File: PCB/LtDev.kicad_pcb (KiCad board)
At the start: 2 copper layers, 90 x 50 mm, 113 parts, among them IC1 TMUX1134PWR, IC2 MMS9013-H-TP, IC3 TPS2116DRLR, IC4 TPS2116DRLR, J1 Conn_JTAG_02x07, J2 Conn_02x05_Odd_Even, J3 Conn_02x05_Odd_Even, J4 Screw_Terminal_01x02, J5 Conn_01x04_Pin, J7 Conn_01x06_Pin, J9 Jumper_Pin_ VIO_CP&3V3, P1 USB_C_Plug (Conv), P2 USB_C_Plug (Prog), SW1 SW_DIP_x02, SW2 SW_DIP_x02, SW3 SW_Push, U1 AMS1117, U2 AMS1117, U3 STM32F103CBTx, U4 CP2102N-Axx-xQFN24, Y1 8MHz

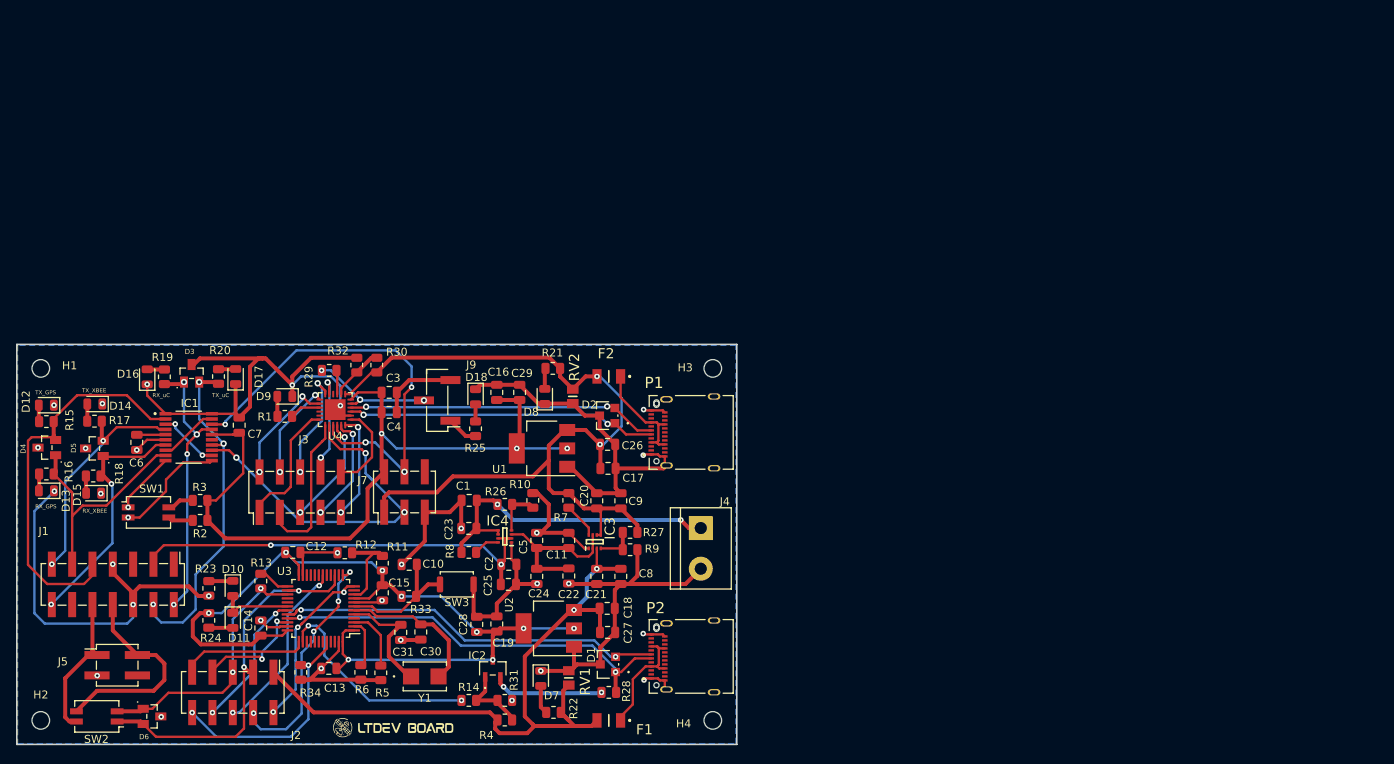
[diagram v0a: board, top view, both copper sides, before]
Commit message: Add files via upload
1.1.0
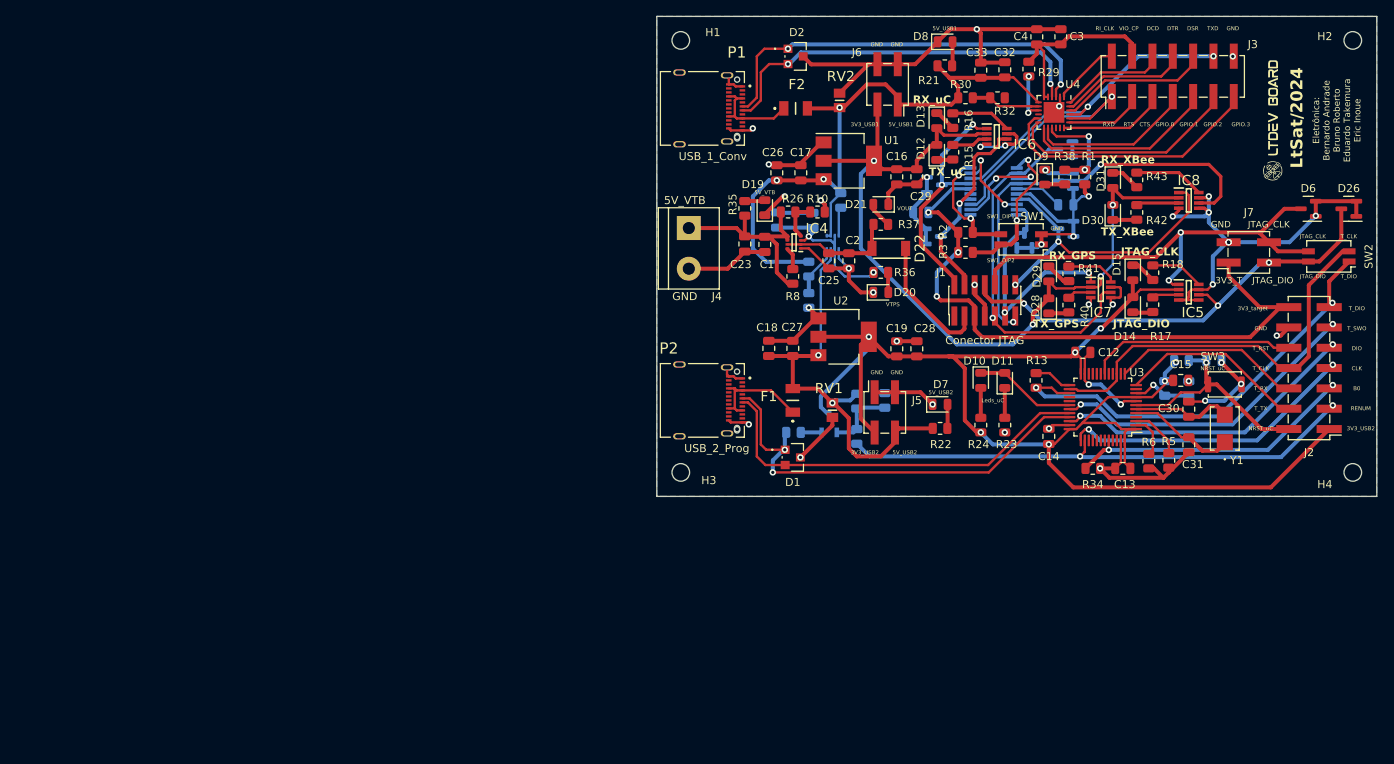
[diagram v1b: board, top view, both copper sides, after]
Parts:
- removed C20, C21, C24: 10uF, Capacitor_SMD:C_0805_2012Metric
- removed C5, C8, C9: 100nF, Capacitor_SMD:C_0805_2012Metric
- removed D16, D17: LED_Green, LED_SMD:LED_0805_2012Metric
- removed D18: LED_Yellow, LED_SMD:LED_0805_2012Metric
- removed J9: Jumper_Pin_ VIO_CP&3V3, Connector_PinHeader_2.54mm:PinHeader_1x03_P2.54mm_Vertical_SMD_Pin1Left
- removed R19, R20: 100R, Resistor_SMD:R_0805_2012Metric
- removed R25: 220R, Resistor_SMD:R_0805_2012Metric
- added C32: 100nF, Capacitor_SMD:C_0805_2012Metric, F.Cu at (179.0, 36.7)
- added C33: 4.7uF, Capacitor_SMD:C_0805_2012Metric, F.Cu at (176.0, 36.7)
- added D19: LED_Red, LED_SMD:LED_0805_2012Metric, F.Cu at (149.0, 53.9)
- added D20: LED_Red, LED_SMD:LED_0805_2012Metric, F.Cu at (163.5, 64.5)
- added D21: LED_Red, LED_SMD:LED_0805_2012Metric, F.Cu at (163.5, 53.5)
- added D22: CMS04_TE12L,Q,M_, Lt_Dev:SODFL4724X108N, F.Cu at (164.5, 59.0)
- added D23: SLVU2.8-MS, Package_TO_SOT_SMD:SOT-23, B.Cu at (186.6, 56.5)
- added D24: SLVU2.8-MS, Package_TO_SOT_SMD:SOT-23, B.Cu at (186.6, 50.5)
- added D25: SLVU2.8-MS, Package_TO_SOT_SMD:SOT-23, B.Cu at (186.5, 46.6)
- added D26: SLVU2.8-MS, Package_TO_SOT_SMD:SOT-23, F.Cu at (222.0, 54.0)
- added D28: LED_Green, LED_SMD:LED_0805_2012Metric, F.Cu at (184.5, 66.2)
- added D29: LED_Green, LED_SMD:LED_0805_2012Metric, F.Cu at (184.5, 62.2)
- added D30: LED_Green, LED_SMD:LED_0805_2012Metric, F.Cu at (192.5, 54.5)
- added D31: LED_Green, LED_SMD:LED_0805_2012Metric, F.Cu at (192.5, 50.5)
- added IC5: TS3A4742DCNR, Lt_Dev:SOT65P280X145-8N, F.Cu at (202.0, 64.5)
- added IC6: TS3A4741DCNR, Lt_Dev:SOT65P280X145-8N, F.Cu at (178.0, 45.0)
- added IC7: TS3A4741DCNR, Lt_Dev:SOT65P280X145-8N, F.Cu at (191.0, 64.2)
- added IC8: TS3A4741DCNR, Lt_Dev:SOT65P280X145-8N, F.Cu at (202.0, 53.0)
- added J6: Conn_02x02_Odd_Even, Connector_PinSocket_2.54mm:PinSocket_2x02_P2.54mm_Vertical_SMD, F.Cu at (164.3, 38.5)
- added R35: 120R, Resistor_SMD:R_0805_2012Metric, F.Cu at (146.5, 54.0)
- added R36: 120R, Resistor_SMD:R_0805_2012Metric, F.Cu at (163.5, 62.0)
- added R37: 120R, Resistor_SMD:R_0805_2012Metric, F.Cu at (163.5, 56.0)
- added R38: 100R, Resistor_SMD:R_0805_2012Metric, F.Cu at (186.5, 50.1)
- added R40: 100R, Resistor_SMD:R_0805_2012Metric, F.Cu at (187.0, 66.1)
- added R41: 100R, Resistor_SMD:R_0805_2012Metric, F.Cu at (187.0, 62.2)
- added R42: 100R, Resistor_SMD:R_0805_2012Metric, F.Cu at (195.5, 54.5)
- added R43: 100R, Resistor_SMD:R_0805_2012Metric, F.Cu at (195.5, 50.4)
- C10, C11, C22, C6, C7, IC1, IC2, IC3, R11, R12, R14, R27, R28, R31, R33, R4, R7, R9: moved to B.Cu
- C4: value 100nF -> 4.7uF
- D10, D9: value LED_Red -> LED_Yellow
- D11: value LED_Yellow -> LED_Red
- D3, D4, D5: value PESD3V3S2UAT,215 -> SLVU2.8-MS; footprint Lt_Dev:SOT95P230X110-3N -> Package_TO_SOT_SMD:SOT-23; moved to B.Cu
- D6: value PESD3V3S2UAT,215 -> SLVU2.8-MS; footprint Lt_Dev:SOT95P230X110-3N -> Package_TO_SOT_SMD:SOT-23
- J1: footprint Connector_PinHeader_2.54mm:PinHeader_2x07_P2.54mm_Vertical_SMD -> Connector_PinHeader_1.27mm:PinHeader_2x07_P1.27mm_Vertical_SMD
- J2, J3: value Conn_02x05_Odd_Even -> Conn_JTAG_02x07; footprint Connector_PinHeader_2.54mm:PinHeader_2x05_P2.54mm_Vertical_SMD -> Connector_PinHeader_2.54mm:PinHeader_2x07_P2.54mm_Vertical_SMD
- J5: value Conn_01x04_Pin -> Conn_02x02_Odd_Even; footprint Connector_PinHeader_2.54mm:PinHeader_2x02_P2.54mm_Vertical_SMD -> Connector_PinSocket_2.54mm:PinSocket_2x02_P2.54mm_Vertical_SMD
- J7: value Conn_01x06_Pin -> Conn_02x02_Odd_Even; footprint Connector_PinHeader_2.54mm:PinHeader_2x03_P2.54mm_Vertical_SMD -> Connector_PinSocket_2.54mm:PinSocket_2x02_P2.54mm_Vertical_SMD
- R29: value 2k -> 1k
- moved H2 184.7 mm to (222.5, 33.0)
- moved SW2 164.4 mm to (219.5, 60.0)
- moved D6 157.9 mm to (216.9, 54.0), turned to 180 degrees
- moved J2 140.5 mm to (217.0, 74.0), turned to 180 degrees
- moved R18 134.9 mm to (197.5, 62.0), turned to 90 degrees
- moved G*** 133.7 mm to (212.5, 43.5), turned to 90 degrees
- moved R17 133.1 mm to (197.5, 66.0), turned to 90 degrees
- moved D15 132.8 mm to (195.0, 62.0), turned to -90 degrees
- moved D14 130.3 mm to (195.0, 66.0), turned to 90 degrees
- moved R16 121.6 mm to (172.5, 43.0), turned to 90 degrees
- moved J3 120.8 mm to (200.0, 37.5)
- moved D13 120.5 mm to (170.5, 43.0), turned to -90 degrees
- moved C6 119.9 mm to (186.6, 53.5), turned to 0 degrees
- moved D5 119.1 mm to (181.4, 58.0)
- moved R15 118.2 mm to (172.5, 47.0), turned to 90 degrees
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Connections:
- C10 pad 1: /NRST -> /NRST_uC
- C3 pad 1: /3V3_USB1 -> /VIO_CP
- C3 pad 2: Net-(J9-Pin_3) -> GND
- C4 pad 1: /3V3_USB1 -> /VIO_CP
- C4 pad 2: Net-(J9-Pin_3) -> GND
- C7 pad 1: /3V3_USB1 -> /3V3_target
- D10 pad 1: Net-(D10-K) -> /LED
- D10 pad 2: /LED -> Net-(D10-A)
- D11 pad 1: /LED -> Net-(D11-K)
- D11 pad 2: Net-(D11-A) -> /LED
- D12 pad 1: GND -> Net-(D12-K)
- D12 pad 2: Net-(D12-A) -> /3V3_USB1
- D13 pad 1: GND -> Net-(D13-K)
- D13 pad 2: Net-(D13-A) -> /3V3_USB1
- D14 pad 1: GND -> Net-(D14-K)
- D14 pad 2: Net-(D14-A) -> /3V3_USB2
- D15 pad 1: GND -> Net-(D15-K)
- D15 pad 2: Net-(D15-A) -> /3V3_USB2
- D3 pad 1: /RX_uC -> GND
- D3 pad 2: /TX_uC -> GND
- D3 pad 3: GND -> /RX_uC
- D4 pad 1: /RX_GPS -> GND
- D4 pad 2: /TX_GPS -> GND
- D4 pad 3: GND -> /TX_uC
- D5 pad 1: /RX_XBEE -> GND
- D5 pad 2: /TX_XBEE -> GND
- D5 pad 3: GND -> /RX_GPS
- D6 pad 1: /T_DIO -> GND
- D6 pad 2: /T_CLK -> GND
- D6 pad 3: GND -> /JTAG_CLK
- IC1 pad 1: GND -> /SW1_DIP1
- IC1 pad 10: GND -> /SW1_DIP1
- IC1 pad 11: GND -> /SW1_DIP2
- IC1 pad 16: /3V3_USB1 -> /3V3_target
- IC1 pad 20: GND -> /SW1_DIP2
- J1 pad 3: /VOUT -> /VOUT_JTAG
- J1 pad 5: unconnected-(J1-Pin_5-Pad5) -> /3V3_target
- J2 pad 1: /5V_USB2 -> /3V3_USB2
- J2 pad 10: /B0 -> /T_RST
- J2 pad 2: /T_TX -> /NRST_uC
- J2 pad 3: /T_CLK -> /RENUM
- J2 pad 4: /T_RX -> /T_TX
- J2 pad 5: /T_DIO -> /B0
- J2 pad 6: /T_RST -> /T_RX
- J2 pad 7: /DIO -> /CLK
- J2 pad 8: /T_SWO -> /T_CLK
- J2 pad 9: /CLK -> /DIO
- J3 pad 1: /CTS -> /RXD
- J3 pad 10: /RI -> /DSR
- J3 pad 2: /GPIO.0 -> /RI_CLK
- J3 pad 4: /GPIO.1 -> /VIO_CP
- J3 pad 5: /DSR -> /CTS
- J3 pad 6: /GPIO.2 -> /DCD
- J3 pad 7: /DTR -> /GPIO.0
- J3 pad 8: /GPIO.3 -> /DTR
- J3 pad 9: /DCD -> /GPIO.1
- J5 pad 1: /JTAG_CLK -> GND
- J5 pad 2: /JTAG_DIO -> /3V3_USB2
- J5 pad 4: unconnected-(J5-Pin_4-Pad4) -> /5V_USB2
- J7 pad 1: /5V_USB1 -> /3V3_target
- J7 pad 2: /3V3_USB1 -> /JTAG_DIO
- J7 pad 3: /RXD -> GND
- J7 pad 4: /TXD -> /JTAG_CLK
- R1 pad 1: Net-(D9-A) -> GND
- R15 pad 1: Net-(D12-A) -> Net-(D12-K)
- R15 pad 2: /TX_GPS -> Net-(IC6-NO2)
- R16 pad 1: Net-(D13-A) -> Net-(D13-K)
- R16 pad 2: /RX_GPS -> Net-(IC6-NO1)
- R17 pad 1: Net-(D14-A) -> Net-(D14-K)
- R17 pad 2: /TX_XBEE -> Net-(IC5-NC2)
- R18 pad 1: Net-(D15-A) -> Net-(D15-K)
- R18 pad 2: /RX_XBEE -> Net-(IC5-NC1)
- R2 pad 1: /3V3_USB1 -> /3V3_target
- R2 pad 2: Net-(R2-Pad2) -> /SW1_DIP2
- R23 pad 2: Net-(D10-K) -> Net-(D11-K)
- R24 pad 1: Net-(D11-A) -> Net-(D10-A)
- R3 pad 1: /3V3_USB1 -> /3V3_target
- R3 pad 2: Net-(R3-Pad2) -> /SW1_DIP1
- R33 pad 1: /NRST -> /NRST_uC
- SW1 pad 3: Net-(R2-Pad2) -> /SW1_DIP2
- SW1 pad 4: Net-(R3-Pad2) -> /SW1_DIP1
- SW2 pad 1: /T_CLK -> /T_DIO
- SW2 pad 2: /T_DIO -> /T_CLK
- SW2 pad 3: /JTAG_DIO -> /JTAG_CLK
- SW2 pad 4: /JTAG_CLK -> /JTAG_DIO
- SW3 pad 2: /NRST -> /NRST_uC
- U3 pad 7: /NRST -> /NRST_uC
- U4 pad 1: /RI -> /RI_CLK
- U4 pad 6: /3V3_USB1 -> /VIO_CP
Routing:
- net /3V3_target: track 0.00 -> 80.6 mm, vias 0 -> 3
- net /3V3_USB2: track 108.3 -> 179.6 mm, vias 9 -> 7
- net /JTAG_CLK: track 18.2 -> 58.5 mm, vias 0 -> 2
- net /VOUT: track 54.1 -> 14.4 mm, vias 2 -> 0
- net /RENUM: track 26.9 -> 65.1 mm
- net /5V_USB2: track 89.2 -> 53.1 mm
- net GND: track 330.4 -> 297.8 mm, vias 33 -> 41
- net /JTAG_DIO: track 26.1 -> 58.1 mm, vias 0 -> 3
- net /NRST_uC: track 0.00 -> 28.0 mm, vias 0 -> 1
- net /DIO: track 14.2 -> 38.8 mm
- net /TX_XBEE: track 29.2 -> 53.6 mm
- net /T_DIO: track 32.8 -> 55.7 mm
- net /5V_USB1: track 106.2 -> 83.5 mm, vias 2 -> 3
- net /T_SWO: track 17.3 -> 39.4 mm
- net /CLK: track 16.0 -> 37.1 mm, vias 0 -> 2
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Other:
- board size 90 x 50 mm -> 90 x 60 mm
- board text added: "3V3_T"
- board text added: "3V3_USB1"
- board text added: "3V3_USB2"
- board text added: "3V3_target"
- board text added: "5V_USB1"
- board text added: "5V_USB2"
- board text added: "5V_VTB"
- board text added: "B0"
- board text added: "CLK"
- board text added: "CTS"
- board text added: "Conector JTAG"
- board text added: "DCD"
- board text added: "DIO"
- board text added: "DSR"
- board text added: "DTR"
- board text added: "Eletrônica: Bernardo Andrade Bruno Roberto Eduardo Takemura Eric Inoue"
- board text added: "GND"
- board text added: "GPIO.0"
- board text added: "GPIO.1"
- board text added: "GPIO.2"
- board text added: "GPIO.3"
- board text added: "JTAG_CLK"
- board text added: "JTAG_DIO"
- board text added: "Leds_uC"
- board text added: "LtSat/2024"
- board text added: "NRST_uC"
- board text added: "RENUM"
- board text added: "RI_CLK"
- board text added: "RTS"
- board text added: "RXD"
- board text added: "RX_XBee"
- board text added: "SW1_DIP1"
- board text added: "SW1_DIP2"
- board text added: "TXD"
- board text added: "TX_XBee"
- board text added: "T_CLK"
- board text added: "T_DIO"
- board text added: "T_RST"
- board text added: "T_RX"
- board text added: "T_SWO"
- board text added: "T_TX"
- board text added: "USB_1_Conv"
- board text added: "USB_2_Prog"
- board text added: "VIO_CP"
- board text added: "VOUT"
- board text added: "VTPS"
- board text removed: "RX_XBEE"
- board text removed: "TX_XBEE"
